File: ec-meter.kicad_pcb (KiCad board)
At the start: 2 copper layers, 46.5 x 56.5 mm, 41 parts, among them P1 Probe, P2 V+, P3 OUT, P4 V-, U1 LM324, U2 LM324

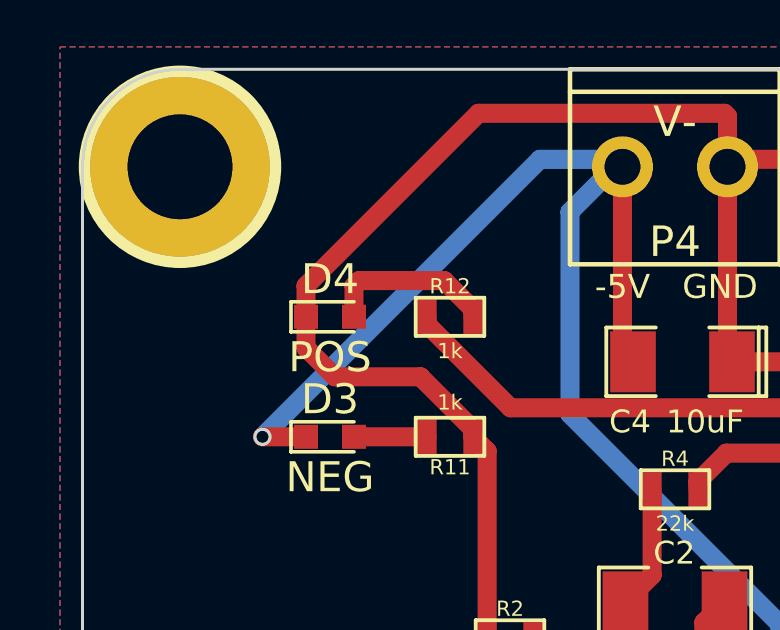
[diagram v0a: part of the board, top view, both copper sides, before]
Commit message: final routing
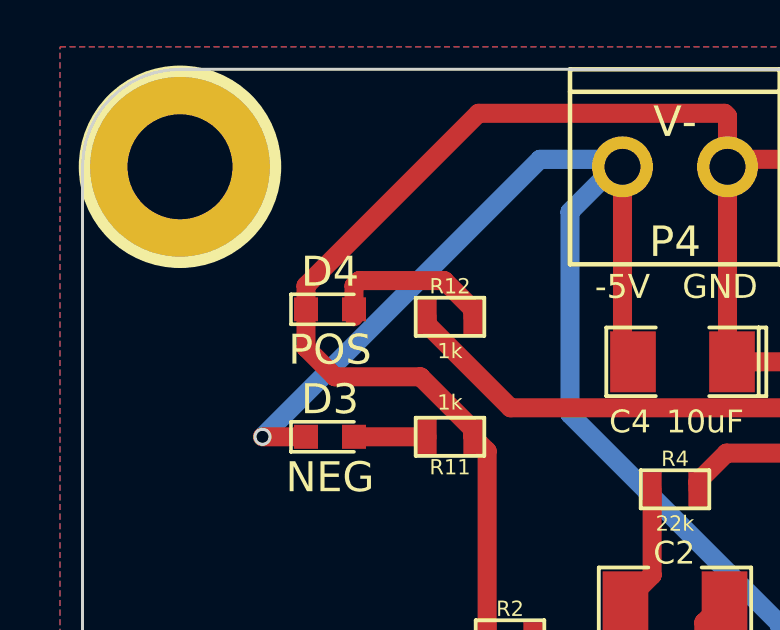
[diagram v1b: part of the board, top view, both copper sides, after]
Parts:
- moved D4 0.25 mm to (35.0, 29.8)
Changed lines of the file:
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@@
     (links 69)
     (no_connects 0)
-    (area 26.699999 21.699999 73.300001 78.300001)
+    (area 22.899999 20.899999 74.100001 81.100001)
     (thickness 1.6)
     (drawings 23)
@@
   )
   (module LEDs:LED_0603 (layer F.Cu)
-    (at 35 30)
+    (at 35 29.75)
     (descr "LED 0603 smd package")
     (tags "LED led 0603 SMD smd SMT smt smdled SMDLED smtled SMTLED")
